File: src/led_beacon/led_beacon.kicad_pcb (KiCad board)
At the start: 2 copper layers, 155 x 40 mm, 0 parts

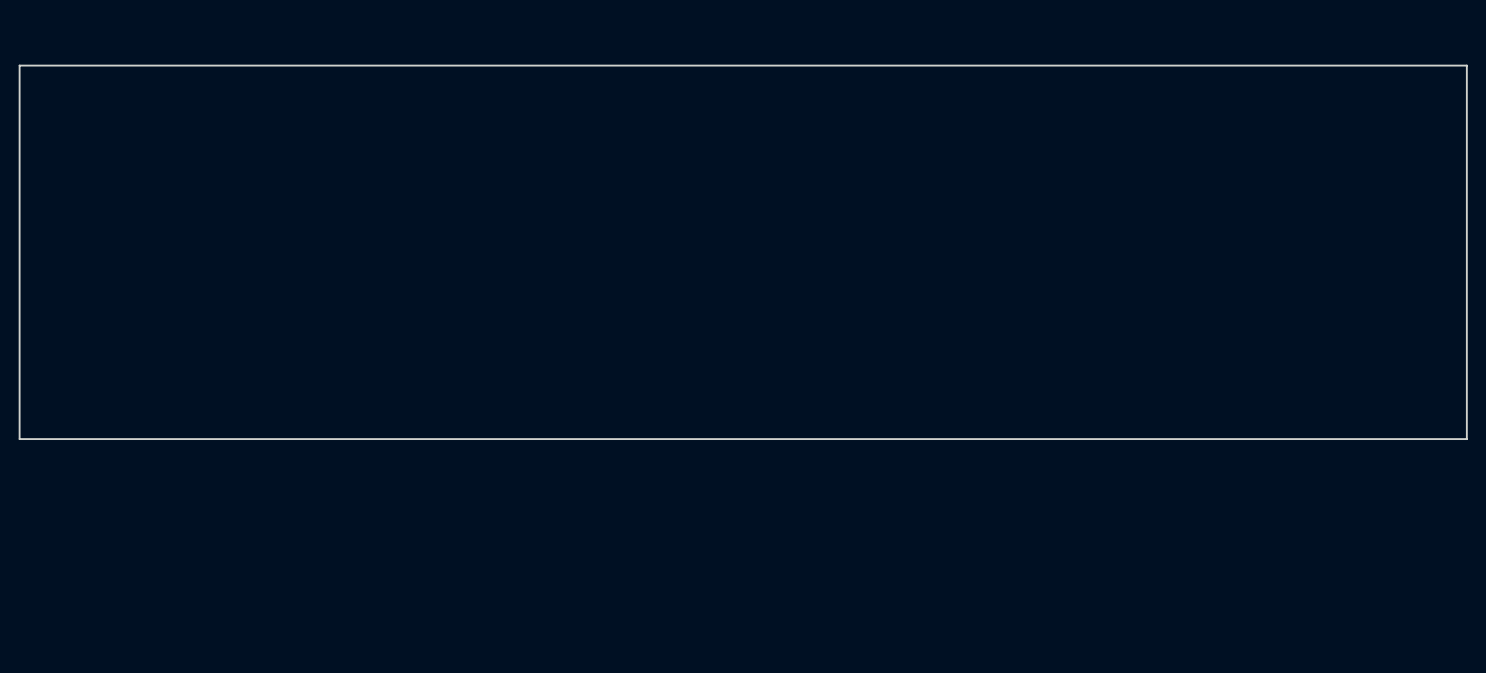
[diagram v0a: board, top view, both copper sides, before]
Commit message: LED Beacon finished
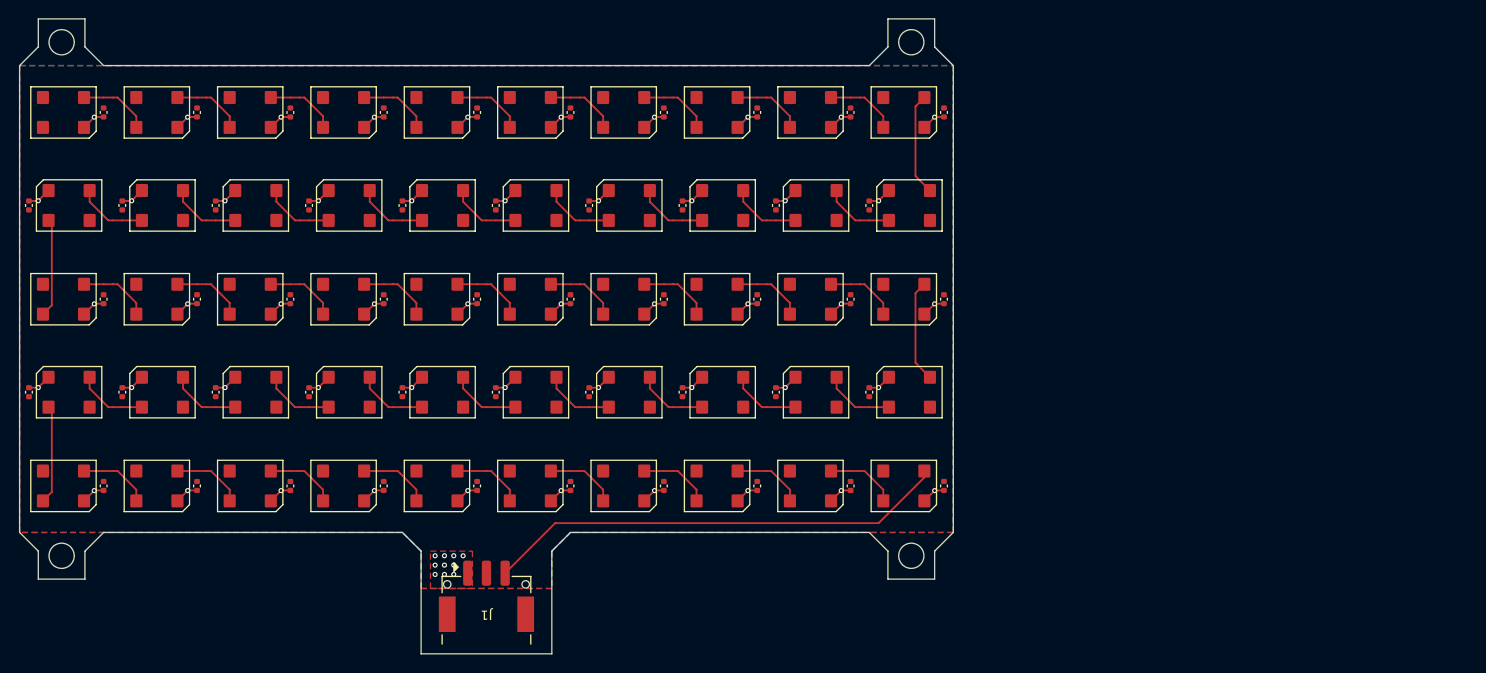
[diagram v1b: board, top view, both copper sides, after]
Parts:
- added C1: 220n, Capacitor_SMD:C_0402_1005Metric, F.Cu at (169.0, 125.0)
- added C10: 220n, Capacitor_SMD:C_0402_1005Metric, F.Cu at (79.0, 125.0)
- added C11: 220n, Capacitor_SMD:C_0402_1005Metric, F.Cu at (71.0, 115.0)
- added C12: 220n, Capacitor_SMD:C_0402_1005Metric, F.Cu at (81.0, 115.0)
- added C13: 220n, Capacitor_SMD:C_0402_1005Metric, F.Cu at (91.0, 115.0)
- added C14: 220n, Capacitor_SMD:C_0402_1005Metric, F.Cu at (101.0, 115.0)
- added C15: 220n, Capacitor_SMD:C_0402_1005Metric, F.Cu at (111.0, 115.0)
- added C16: 220n, Capacitor_SMD:C_0402_1005Metric, F.Cu at (121.0, 115.0)
- added C17: 220n, Capacitor_SMD:C_0402_1005Metric, F.Cu at (131.0, 115.0)
- added C18: 220n, Capacitor_SMD:C_0402_1005Metric, F.Cu at (141.0, 115.0)
- added C19: 220n, Capacitor_SMD:C_0402_1005Metric, F.Cu at (151.0, 115.0)
- added C2: 220n, Capacitor_SMD:C_0402_1005Metric, F.Cu at (159.0, 125.0)
- added C20: 220n, Capacitor_SMD:C_0402_1005Metric, F.Cu at (161.0, 115.0)
- added C21: 220n, Capacitor_SMD:C_0402_1005Metric, F.Cu at (169.0, 105.0)
- added C22: 220n, Capacitor_SMD:C_0402_1005Metric, F.Cu at (159.0, 105.0)
- added C23: 220n, Capacitor_SMD:C_0402_1005Metric, F.Cu at (149.0, 105.0)
- added C24: 220n, Capacitor_SMD:C_0402_1005Metric, F.Cu at (139.0, 105.0)
- added C25: 220n, Capacitor_SMD:C_0402_1005Metric, F.Cu at (129.0, 105.0)
- added C26: 220n, Capacitor_SMD:C_0402_1005Metric, F.Cu at (119.0, 105.0)
- added C27: 220n, Capacitor_SMD:C_0402_1005Metric, F.Cu at (109.0, 105.0)
- added C28: 220n, Capacitor_SMD:C_0402_1005Metric, F.Cu at (99.0, 105.0)
- added C29: 220n, Capacitor_SMD:C_0402_1005Metric, F.Cu at (89.0, 105.0)
- added C3: 220n, Capacitor_SMD:C_0402_1005Metric, F.Cu at (149.0, 125.0)
- added C30: 220n, Capacitor_SMD:C_0402_1005Metric, F.Cu at (79.0, 105.0)
- added C31: 220n, Capacitor_SMD:C_0402_1005Metric, F.Cu at (71.0, 95.0)
- added C32: 220n, Capacitor_SMD:C_0402_1005Metric, F.Cu at (81.0, 95.0)
- added C33: 220n, Capacitor_SMD:C_0402_1005Metric, F.Cu at (91.0, 95.0)
- added C34: 220n, Capacitor_SMD:C_0402_1005Metric, F.Cu at (101.0, 95.0)
- added C35: 220n, Capacitor_SMD:C_0402_1005Metric, F.Cu at (111.0, 95.0)
- added C36: 220n, Capacitor_SMD:C_0402_1005Metric, F.Cu at (121.0, 95.0)
- added C37: 220n, Capacitor_SMD:C_0402_1005Metric, F.Cu at (131.0, 95.0)
- added C38: 220n, Capacitor_SMD:C_0402_1005Metric, F.Cu at (141.0, 95.0)
- added C39: 220n, Capacitor_SMD:C_0402_1005Metric, F.Cu at (151.0, 95.0)
- added C4: 220n, Capacitor_SMD:C_0402_1005Metric, F.Cu at (139.0, 125.0)
- added C40: 220n, Capacitor_SMD:C_0402_1005Metric, F.Cu at (161.0, 95.0)
- added C41: 220n, Capacitor_SMD:C_0402_1005Metric, F.Cu at (169.0, 85.0)
- added C42: 220n, Capacitor_SMD:C_0402_1005Metric, F.Cu at (159.0, 85.0)
- added C43: 220n, Capacitor_SMD:C_0402_1005Metric, F.Cu at (149.0, 85.0)
- added C44: 220n, Capacitor_SMD:C_0402_1005Metric, F.Cu at (139.0, 85.0)
- added C45: 220n, Capacitor_SMD:C_0402_1005Metric, F.Cu at (129.0, 85.0)
- added C46: 220n, Capacitor_SMD:C_0402_1005Metric, F.Cu at (119.0, 85.0)
- added C47: 220n, Capacitor_SMD:C_0402_1005Metric, F.Cu at (109.0, 85.0)
- added C48: 220n, Capacitor_SMD:C_0402_1005Metric, F.Cu at (99.0, 85.0)
- added C49: 220n, Capacitor_SMD:C_0402_1005Metric, F.Cu at (89.0, 85.0)
- added C5: 220n, Capacitor_SMD:C_0402_1005Metric, F.Cu at (129.0, 125.0)
- added C50: 220n, Capacitor_SMD:C_0402_1005Metric, F.Cu at (79.0, 85.0)
- added C6: 220n, Capacitor_SMD:C_0402_1005Metric, F.Cu at (119.0, 125.0)
- added C7: 220n, Capacitor_SMD:C_0402_1005Metric, F.Cu at (109.0, 125.0)
- added C8: 220n, Capacitor_SMD:C_0402_1005Metric, F.Cu at (99.0, 125.0)
- added C9: 220n, Capacitor_SMD:C_0402_1005Metric, F.Cu at (89.0, 125.0)
- added D1: WS2812B, Bluesat:WS2812B-5050, F.Cu at (164.7, 125.0)
- added D10: WS2812B, Bluesat:WS2812B-5050, F.Cu at (74.7, 125.0)
- added D11: WS2812B, Bluesat:WS2812B-5050, F.Cu at (75.3, 115.0)
- added D12: WS2812B, Bluesat:WS2812B-5050, F.Cu at (85.3, 115.0)
- added D13: WS2812B, Bluesat:WS2812B-5050, F.Cu at (95.3, 115.0)
- added D14: WS2812B, Bluesat:WS2812B-5050, F.Cu at (105.3, 115.0)
- added D15: WS2812B, Bluesat:WS2812B-5050, F.Cu at (115.3, 115.0)
- added D16: WS2812B, Bluesat:WS2812B-5050, F.Cu at (125.3, 115.0)
- added D17: WS2812B, Bluesat:WS2812B-5050, F.Cu at (135.3, 115.0)
- added D18: WS2812B, Bluesat:WS2812B-5050, F.Cu at (145.3, 115.0)
- added D19: WS2812B, Bluesat:WS2812B-5050, F.Cu at (155.3, 115.0)
- added D2: WS2812B, Bluesat:WS2812B-5050, F.Cu at (154.7, 125.0)
- added D20: WS2812B, Bluesat:WS2812B-5050, F.Cu at (165.3, 115.0)
- added D21: WS2812B, Bluesat:WS2812B-5050, F.Cu at (164.7, 105.0)
- added D22: WS2812B, Bluesat:WS2812B-5050, F.Cu at (154.7, 105.0)
- added D23: WS2812B, Bluesat:WS2812B-5050, F.Cu at (144.7, 105.0)
- added D24: WS2812B, Bluesat:WS2812B-5050, F.Cu at (134.7, 105.0)
- added D25: WS2812B, Bluesat:WS2812B-5050, F.Cu at (124.7, 105.0)
- added D26: WS2812B, Bluesat:WS2812B-5050, F.Cu at (114.7, 105.0)
- added D27: WS2812B, Bluesat:WS2812B-5050, F.Cu at (104.7, 105.0)
- added D28: WS2812B, Bluesat:WS2812B-5050, F.Cu at (94.7, 105.0)
- added D29: WS2812B, Bluesat:WS2812B-5050, F.Cu at (84.7, 105.0)
- added D3: WS2812B, Bluesat:WS2812B-5050, F.Cu at (144.7, 125.0)
- added D30: WS2812B, Bluesat:WS2812B-5050, F.Cu at (74.7, 105.0)
- added D31: WS2812B, Bluesat:WS2812B-5050, F.Cu at (75.3, 95.0)
- added D32: WS2812B, Bluesat:WS2812B-5050, F.Cu at (85.3, 95.0)
- added D33: WS2812B, Bluesat:WS2812B-5050, F.Cu at (95.3, 95.0)
- added D34: WS2812B, Bluesat:WS2812B-5050, F.Cu at (105.3, 95.0)
- added D35: WS2812B, Bluesat:WS2812B-5050, F.Cu at (115.3, 95.0)
- added D36: WS2812B, Bluesat:WS2812B-5050, F.Cu at (125.3, 95.0)
- added D37: WS2812B, Bluesat:WS2812B-5050, F.Cu at (135.3, 95.0)
- added D38: WS2812B, Bluesat:WS2812B-5050, F.Cu at (145.3, 95.0)
- added D39: WS2812B, Bluesat:WS2812B-5050, F.Cu at (155.3, 95.0)
- added D4: WS2812B, Bluesat:WS2812B-5050, F.Cu at (134.7, 125.0)
- added D40: WS2812B, Bluesat:WS2812B-5050, F.Cu at (165.3, 95.0)
- added D41: WS2812B, Bluesat:WS2812B-5050, F.Cu at (164.7, 85.0)
- added D42: WS2812B, Bluesat:WS2812B-5050, F.Cu at (154.7, 85.0)
- added D43: WS2812B, Bluesat:WS2812B-5050, F.Cu at (144.7, 85.0)
- added D44: WS2812B, Bluesat:WS2812B-5050, F.Cu at (134.7, 85.0)
- added D45: WS2812B, Bluesat:WS2812B-5050, F.Cu at (124.7, 85.0)
- added D46: WS2812B, Bluesat:WS2812B-5050, F.Cu at (114.7, 85.0)
- added D47: WS2812B, Bluesat:WS2812B-5050, F.Cu at (104.7, 85.0)
- added D48: WS2812B, Bluesat:WS2812B-5050, F.Cu at (94.7, 85.0)
- added D49: WS2812B, Bluesat:WS2812B-5050, F.Cu at (84.7, 85.0)
- added D5: WS2812B, Bluesat:WS2812B-5050, F.Cu at (124.7, 125.0)
- added D50: WS2812B, Bluesat:WS2812B-5050, F.Cu at (74.7, 85.0)
- added D6: WS2812B, Bluesat:WS2812B-5050, F.Cu at (114.7, 125.0)
- added D7: WS2812B, Bluesat:WS2812B-5050, F.Cu at (104.7, 125.0)
- added D8: WS2812B, Bluesat:WS2812B-5050, F.Cu at (94.7, 125.0)
- added D9: WS2812B, Bluesat:WS2812B-5050, F.Cu at (84.7, 125.0)
- added H1: M2.5, Bluesat:M2.5_Internal, F.Cu at (74.5, 132.5)
- added H2: M2.5, Bluesat:M2.5_Internal, F.Cu at (165.5, 132.5)
- added H3: M2.5, Bluesat:M2.5_Internal, F.Cu at (74.5, 77.5)
- added H4: M2.5, Bluesat:M2.5_Internal, F.Cu at (165.5, 77.5)
- added J1: Conn_01x03, Bluesat:SM03B-PASS, F.Cu at (120.0, 142.5)
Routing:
- net GND: track 0.00 -> 128.2 mm, vias 0 -> 60
- net Net-(D1-DIN): track 0.00 -> 49.8 mm
- net Net-(D40-DOUT): track 0.00 -> 11.0 mm
- net Net-(D20-DOUT): track 0.00 -> 11.0 mm
- net Net-(D30-DOUT): track 0.00 -> 10.6 mm
- net Net-(D10-DOUT): track 0.00 -> 10.6 mm
- net Net-(D8-DOUT): track 0.00 -> 7.63 mm
- net Net-(D7-DOUT): track 0.00 -> 7.63 mm
- net Net-(D6-DOUT): track 0.00 -> 7.63 mm
- net Net-(D5-DOUT): track 0.00 -> 7.63 mm
- net Net-(D49-DOUT): track 0.00 -> 7.63 mm
- net Net-(D48-DOUT): track 0.00 -> 7.63 mm
- net Net-(D47-DOUT): track 0.00 -> 7.63 mm
- net Net-(D46-DOUT): track 0.00 -> 7.63 mm
- net Net-(D45-DOUT): track 0.00 -> 7.63 mm
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- added copper zone on F.Cu, net +5V
- added copper zone on B.Cu, net GND
- added copper zone on F.Cu, net GND
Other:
- board size 155 x 40 mm -> 100 x 68 mm
